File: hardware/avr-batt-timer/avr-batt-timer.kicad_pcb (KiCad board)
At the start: 2 copper layers, 25.5 x 56.9 mm, 13 parts, among them J1 XT60PW-M, J2 XT60PW-F, J3 Conn_01x05_Pin, U1 ATtiny5-TS, U2 L78L05_SOT89

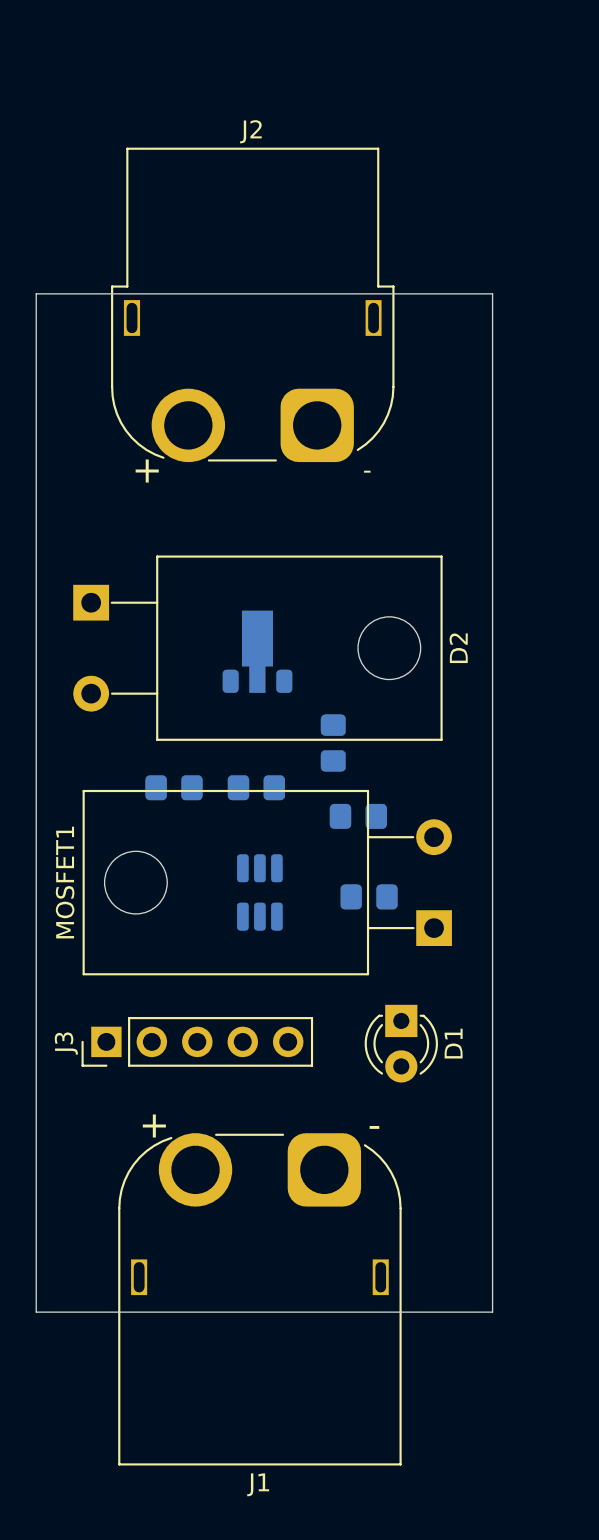
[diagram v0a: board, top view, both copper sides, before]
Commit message: +1
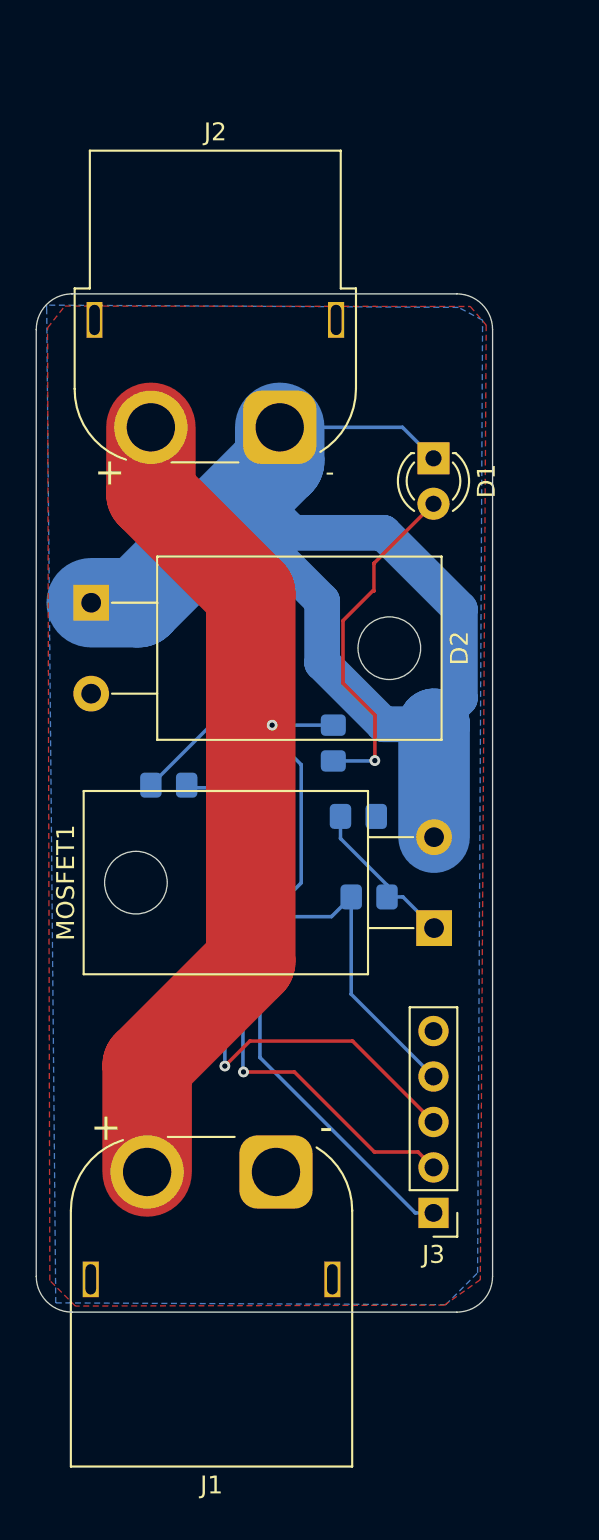
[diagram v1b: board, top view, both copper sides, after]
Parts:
- moved D1 31.5 mm to (149.1, 72.4)
- moved J3 20.6 mm to (149.1, 114.6), turned to 180 degrees
- moved J1 2.71 mm to (140.3, 112.3)
- moved J2 2.10 mm to (140.5, 70.7)
- moved R1 0.33 mm to (134.3, 90.7), turned to 0 degrees
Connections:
- R1 pad 1: VCC -> VDD
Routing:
- net LOAD: track 0.00 -> 71.4 mm
- net VDD: track 0.00 -> 57.4 mm, vias 0 -> 1
- net +5V: track 0.00 -> 39.6 mm
- net TPIDATA: track 0.00 -> 25.6 mm, vias 0 -> 1
- net RESET: track 0.00 -> 21.5 mm, vias 0 -> 1
- net Net-(D1-A): track 0.00 -> 19.6 mm, vias 0 -> 1
- net TPICLK: track 0.00 -> 16.5 mm
- net Net-(MOSFET1-G): track 0.00 -> 8.93 mm
- net VSENSE: track 0.00 -> 8.38 mm
- added copper zone on B.Cu, net GND
- added copper zone on F.Cu, net VDD
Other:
- outline, holes or cut-outs redrawn

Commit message: +1
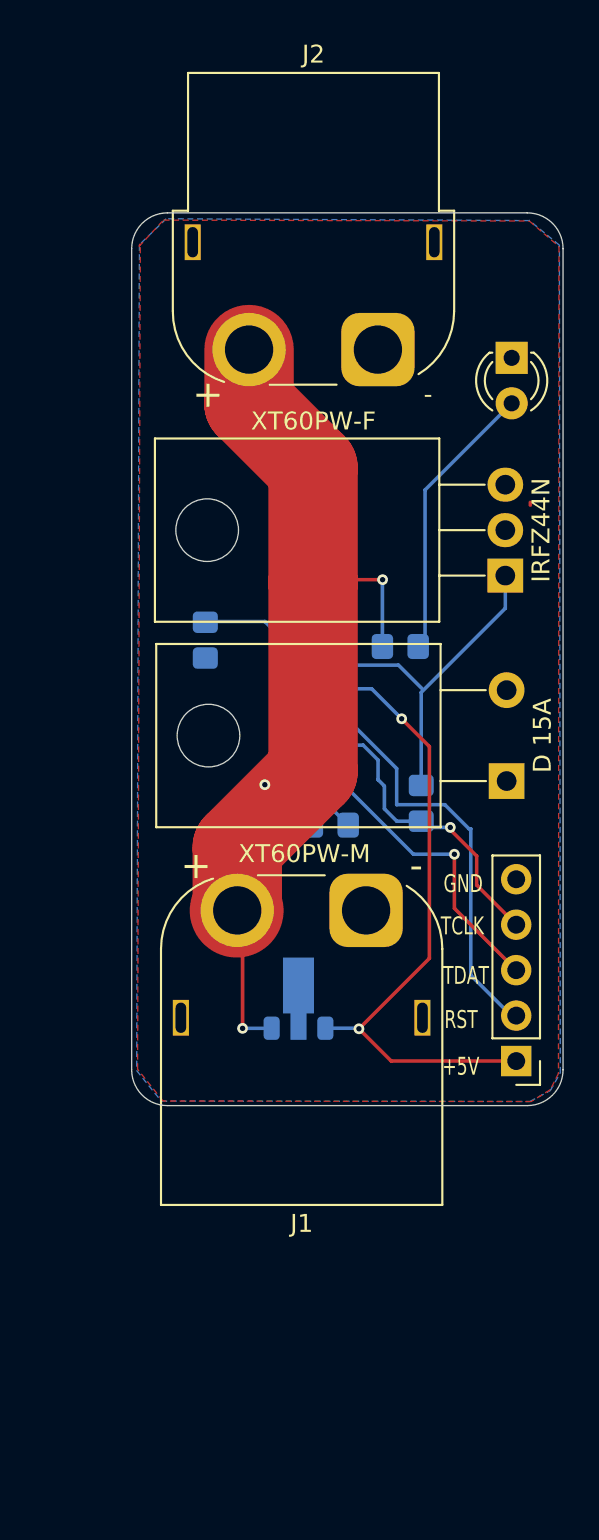
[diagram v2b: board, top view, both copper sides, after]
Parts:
- D2: value D -> D 15A
- MOSFET1: value IRFZ44N_127 -> IRFZ44N; footprint Package_TO_SOT_THT:TO-220-2_Horizontal_TabDown -> Package_TO_SOT_THT:TO-220-3_Horizontal_TabDown
- R3: value ~ 250R -> ~250R
- R4: value ~ 10K -> ~10K
- R5: value ~ 700R -> ~700R
- U1: value ATtiny5-TS -> ATtiny5
- moved D2 25.3 mm to (153.2, 90.4), turned to 90 degrees
- moved MOSFET1 20.1 mm to (153.1, 78.9)
- moved U2 19.5 mm to (141.6, 102.3)
- moved J1 15.5 mm to (145.3, 97.7)
- moved R4 13.0 mm to (136.3, 82.5), turned to -90 degrees
- moved J3 9.66 mm to (153.7, 106.1)
- moved U1 9.16 mm to (143.5, 88.4), turned to 90 degrees
- moved D1 7.11 mm to (153.5, 66.8)
- moved J2 7.00 mm to (146.0, 66.3)
- moved R5 6.57 mm to (147.2, 82.9), turned to 0 degrees
- moved R3 5.99 mm to (148.4, 91.7), turned to -90 degrees
- moved R1 5.33 mm to (139.1, 92.9)
- moved R2 4.63 mm to (143.3, 92.9)
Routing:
- net LOAD: track 71.4 -> 0.15 mm
- net Net-(MOSFET1-G): track 8.93 -> 27.8 mm
- net TPIDATA: track 25.6 -> 16.4 mm
- net Net-(D1-A): track 19.6 -> 15.2 mm, vias 1 -> 0
- net VDD: track 57.4 -> 53.1 mm, vias 1 -> 3
- net GND: track 0.00 -> 3.46 mm
- net VSENSE: track 8.38 -> 5.09 mm
- net +5V: track 39.6 -> 37.3 mm, vias 0 -> 2
- net TPICLK: track 16.5 -> 18.6 mm, vias 0 -> 1
- net RESET: track 21.5 -> 21.8 mm, vias 1 -> 0
- added copper zone on F.Cu, net LOAD
- removed copper zone on F.Cu, net VDD
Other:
- board size 25.5 x 56.9 mm -> 24.1 x 49.9 mm
- board text added: "+5V"
- board text added: "GND"
- board text added: "RST"
- board text added: "TCLK"
- board text added: "TDAT"
